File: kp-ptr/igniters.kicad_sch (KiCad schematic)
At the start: 52 parts, among them J10 Conn_01x02, J11 Conn_01x02, J12 Conn_01x02, J13 Conn_01x02, Q10 PMOS_SOT23, Q11 PMOS_SOT23, Q12 PMOS_SOT23, Q13 PMOS_SOT23, Q2 PMOS_SOT23, Q3 PMOS_SOT23, Q4 PMOS_SOT23, Q5 PMOS_SOT23, Q6 NMOS_SOT23, Q7 NMOS_SOT23, Q8 NMOS_SOT23, Q9 NMOS_SOT23

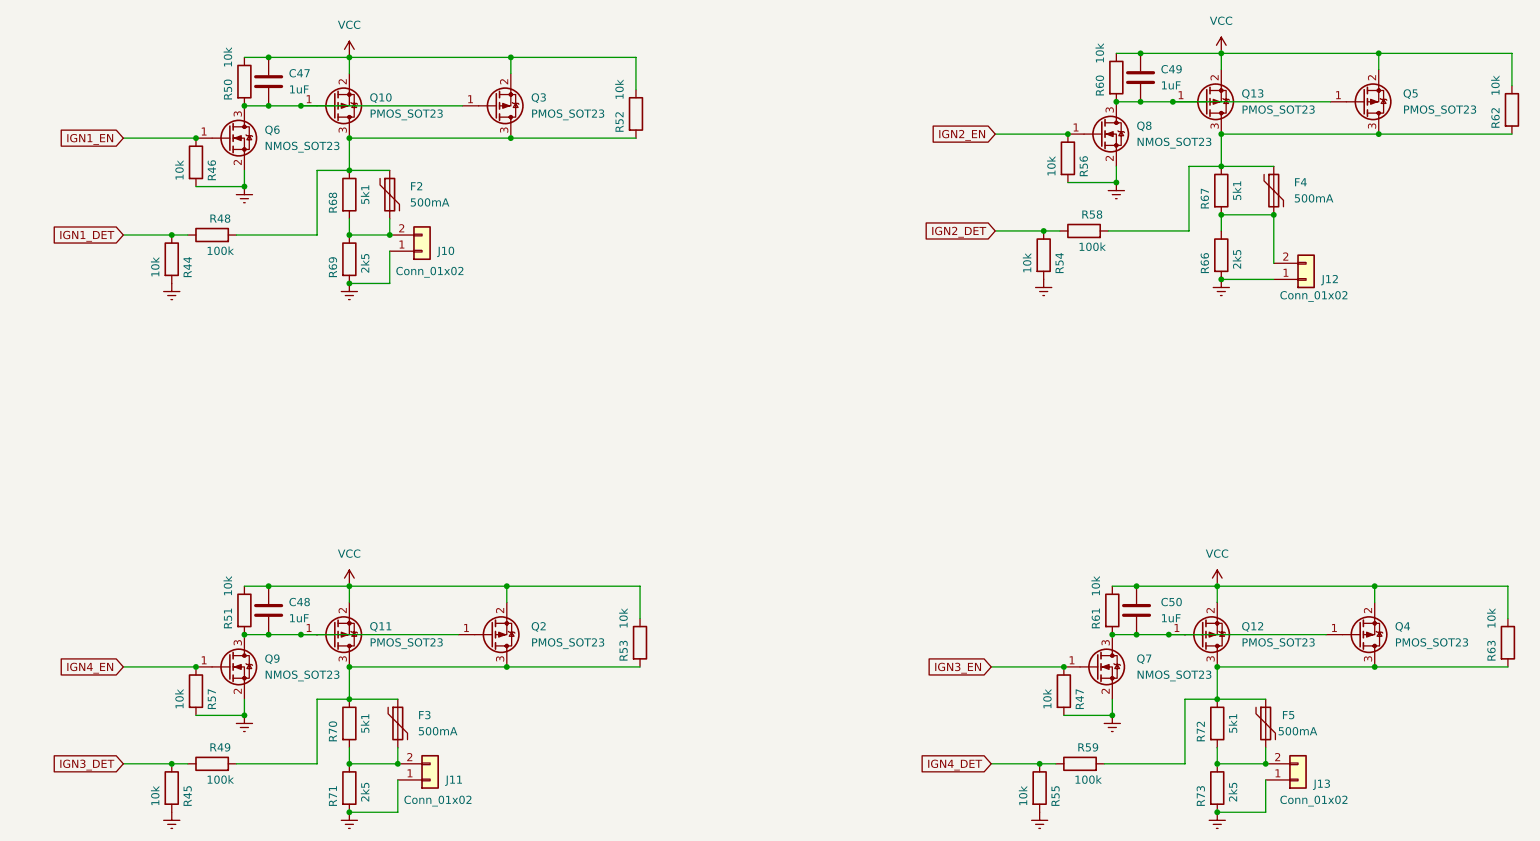
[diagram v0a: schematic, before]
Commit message: Parts renumbered! Noice!
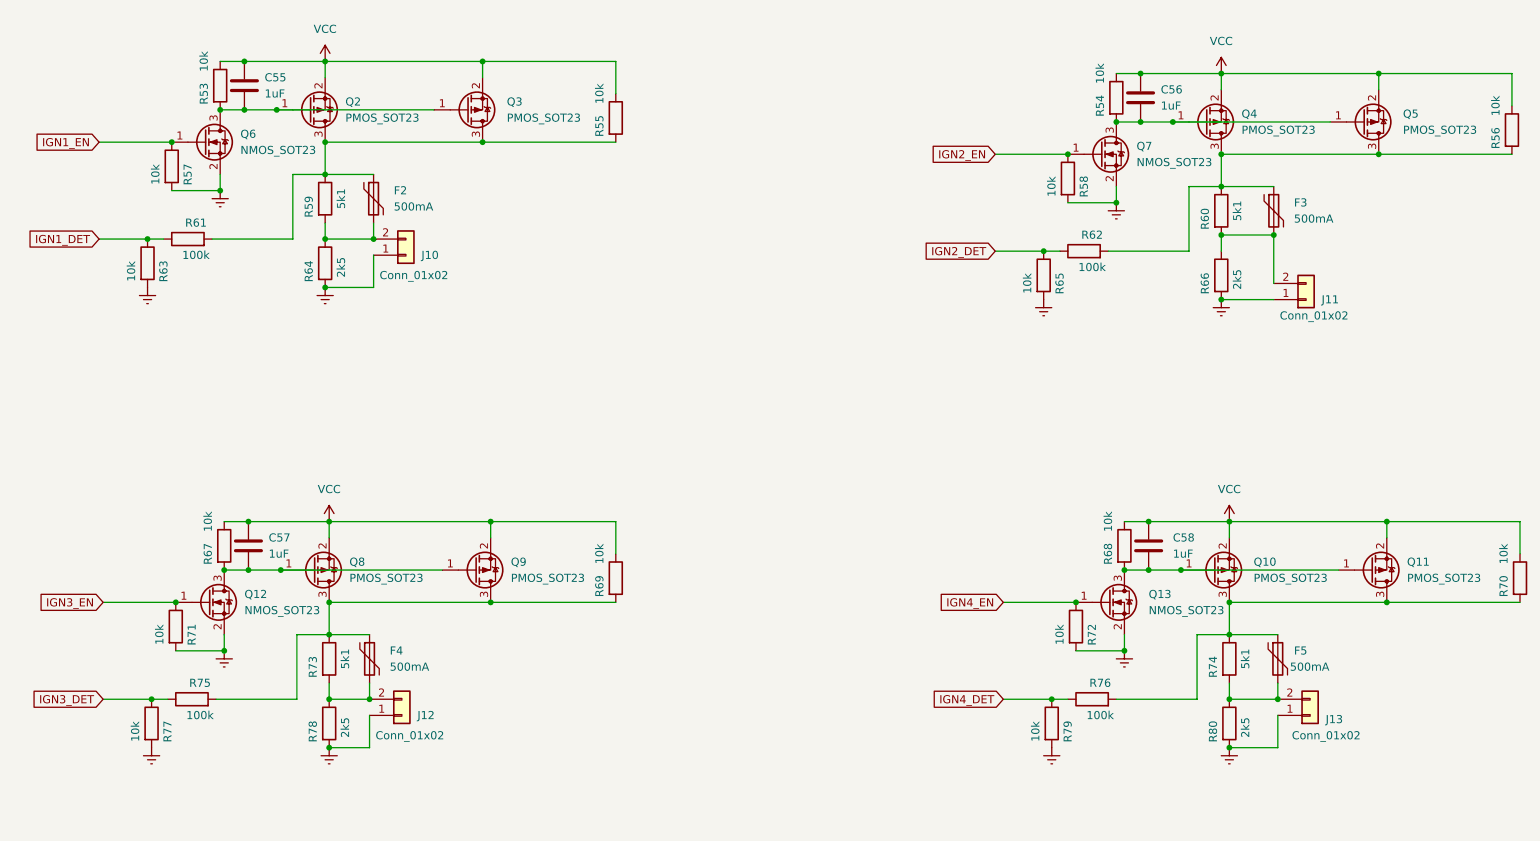
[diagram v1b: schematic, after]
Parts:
- renumbered C48 to C55, C49 to C56, C47 to C57, C50 to C58, F3 to F2, F4 to F3, F2 to F4, J11 to J10, J12 to J11, J10 to J12, Q12 to Q10, Q4 to Q11, Q6 to Q12, Q7 to Q13, Q11 to Q2, Q2 to Q3, Q13 to Q4, Q9 to Q6, Q8 to Q7, Q10 to Q8, Q3 to Q9, R51 to R53, R60 to R54, R53 to R55, R62 to R56, R56 to R58, R70 to R59, R67 to R60, R49 to R61, R58 to R62, R45 to R63, R71 to R64, R54 to R65, R50 to R67, R61 to R68, R52 to R69, R63 to R70, R46 to R71, R47 to R72, R68 to R73, R72 to R74, R48 to R75, R59 to R76, R44 to R77, R69 to R78, R55 to R79, R73 to R80
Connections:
- net IGN1_DET: now also R61.1, R63.1; no longer R75.1, R77.1
- net IGN1_EN: now also Q6.1 (G), R57.1; no longer Q12.1 (G), R71.1
- net IGN3_DET: now also R75.1, R77.1; no longer R61.1, R63.1
- net IGN3_EN: now also Q12.1 (G), R71.1; no longer Q13.1 (G), R72.1
- net IGN4_EN: now also Q13.1 (G), R72.1; no longer Q6.1 (G), R57.1
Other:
- moved on the sheet: C55, C56, C57, C58, F2, F3, F4, F5, J10, J11, J12, J13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
